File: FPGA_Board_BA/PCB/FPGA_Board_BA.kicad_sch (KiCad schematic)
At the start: 4 parts

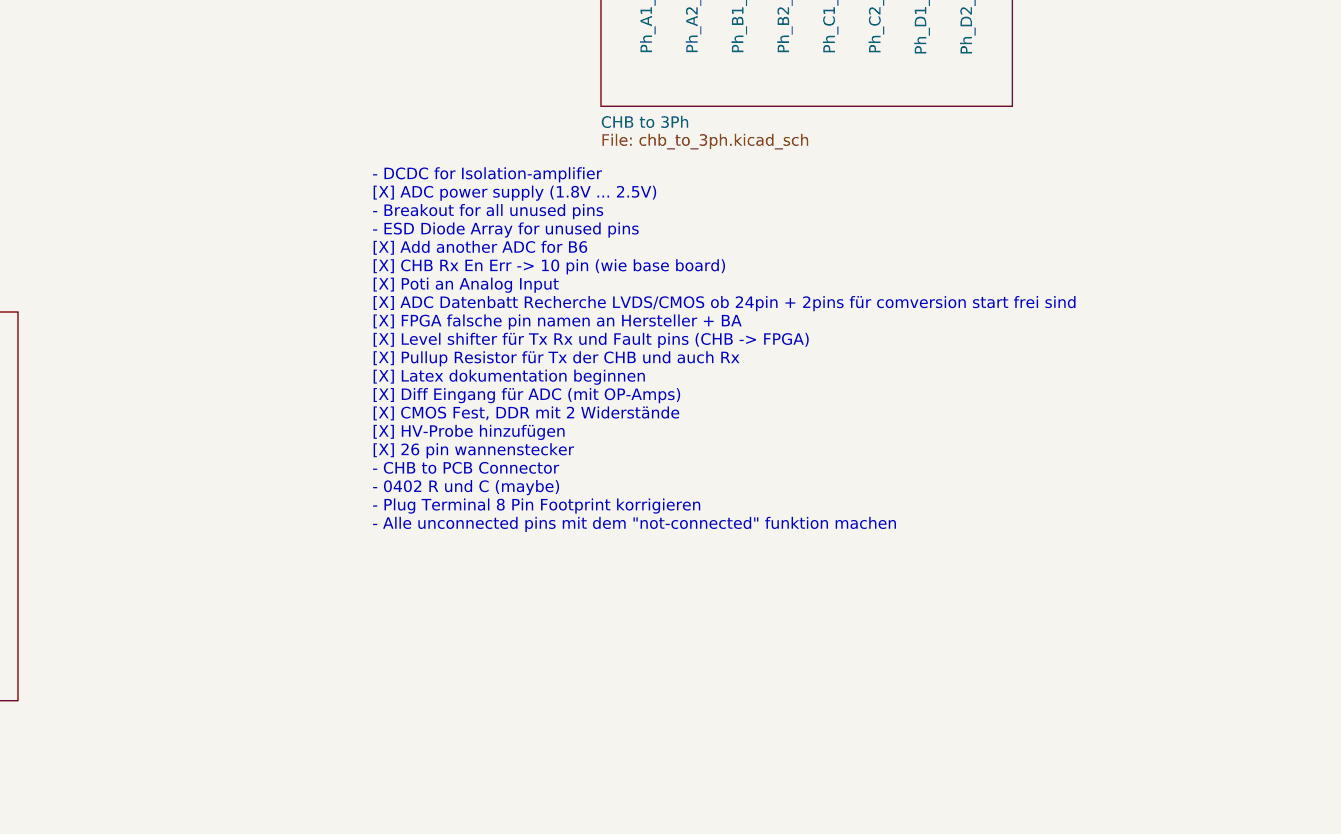
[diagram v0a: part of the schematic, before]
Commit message: Besprechung mit Leo
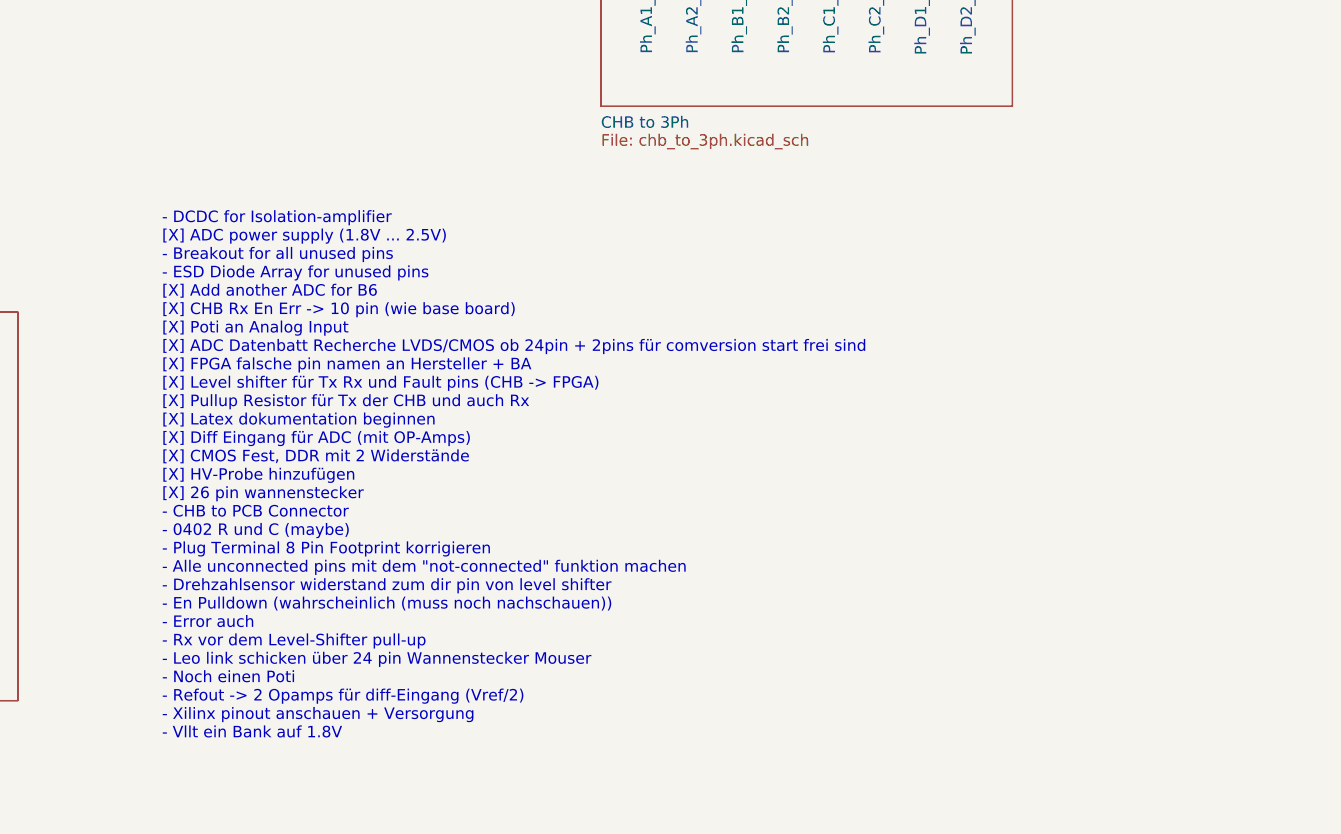
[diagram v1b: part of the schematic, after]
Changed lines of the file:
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@@
 	(generator_version "9.0")
 	(paper "A3")
-	(text "- DCDC for Isolation-amplifier\n[X] ADC power supply (1.8V ... 2.5V)\n- Breakout for all unused pins\n- ESD Diode Array for unused pins\n[X] Add another ADC for B6\n[X] CHB Rx En Err -> 10 pin (wie base board)\n[X] Poti an Analog Input\n[X] ADC Datenbatt Recherche LVDS/CMOS ob 24pin + 2pins für comversion start frei sind\n[X] FPGA falsche pin namen an Hersteller + BA \n[X] Level shifter für Tx Rx und Fault pins (CHB -> FPGA)\n[X] Pullup Resistor für Tx der CHB und auch Rx\n[X] Latex dokumentation beginnen\n[X] Diff Eingang für ADC (mit OP-Amps)\n[X] CMOS Fest, DDR mit 2 Widerstände\n[X] HV-Probe hinzufügen\n[X] 26 pin wannenstecker\n- CHB to PCB Connector \n- 0402 R und C (maybe)\n- Plug Terminal 8 Pin Footprint korrigieren\n- Alle unconnected pins mit dem \"not-connected\" funktion machen"
+	(text "- DCDC for Isolation-amplifier\n[X] ADC power supply (1.8V ... 2.5V)\n- Breakout for all unused pins\n- ESD Diode Array for unused pins\n[X] Add another ADC for B6\n[X] CHB Rx En Err -> 10 pin (wie base board)\n[X] Poti an Analog Input\n[X] ADC Datenbatt Recherche LVDS/CMOS ob 24pin + 2pins für comversion start frei sind\n[X] FPGA falsche pin namen an Hersteller + BA \n[X] Level shifter für Tx Rx und Fault pins (CHB -> FPGA)\n[X] Pullup Resistor für Tx der CHB und auch Rx\n[X] Latex dokumentation beginnen\n[X] Diff Eingang für ADC (mit OP-Amps)\n[X] CMOS Fest, DDR mit 2 Widerstände\n[X] HV-Probe hinzufügen\n[X] 26 pin wannenstecker\n- CHB to PCB Connector \n- 0402 R und C (maybe)\n- Plug Terminal 8 Pin Footprint korrigieren\n- Alle unconnected pins mit dem \"not-connected\" funktion machen\n- Drehzahlsensor widerstand zum dir pin von level shifter\n- En Pulldown (wahrscheinlich (muss noch nachschauen))\n- Error auch\n- Rx vor dem Level-Shifter pull-up\n- Leo link schicken über 24 pin Wannenstecker Mouser\n- Noch einen Poti \n- Refout -> 2 Opamps für diff-Eingang (Vref/2)\n- Xilinx pinout anschauen + Versorgung\n- Vllt ein Bank auf 1.8V"
 		(exclude_from_sim no)
-		(at 302.26 230.378 0)
+		(at 278.892 244.348 0)
 		(effects
 			(font

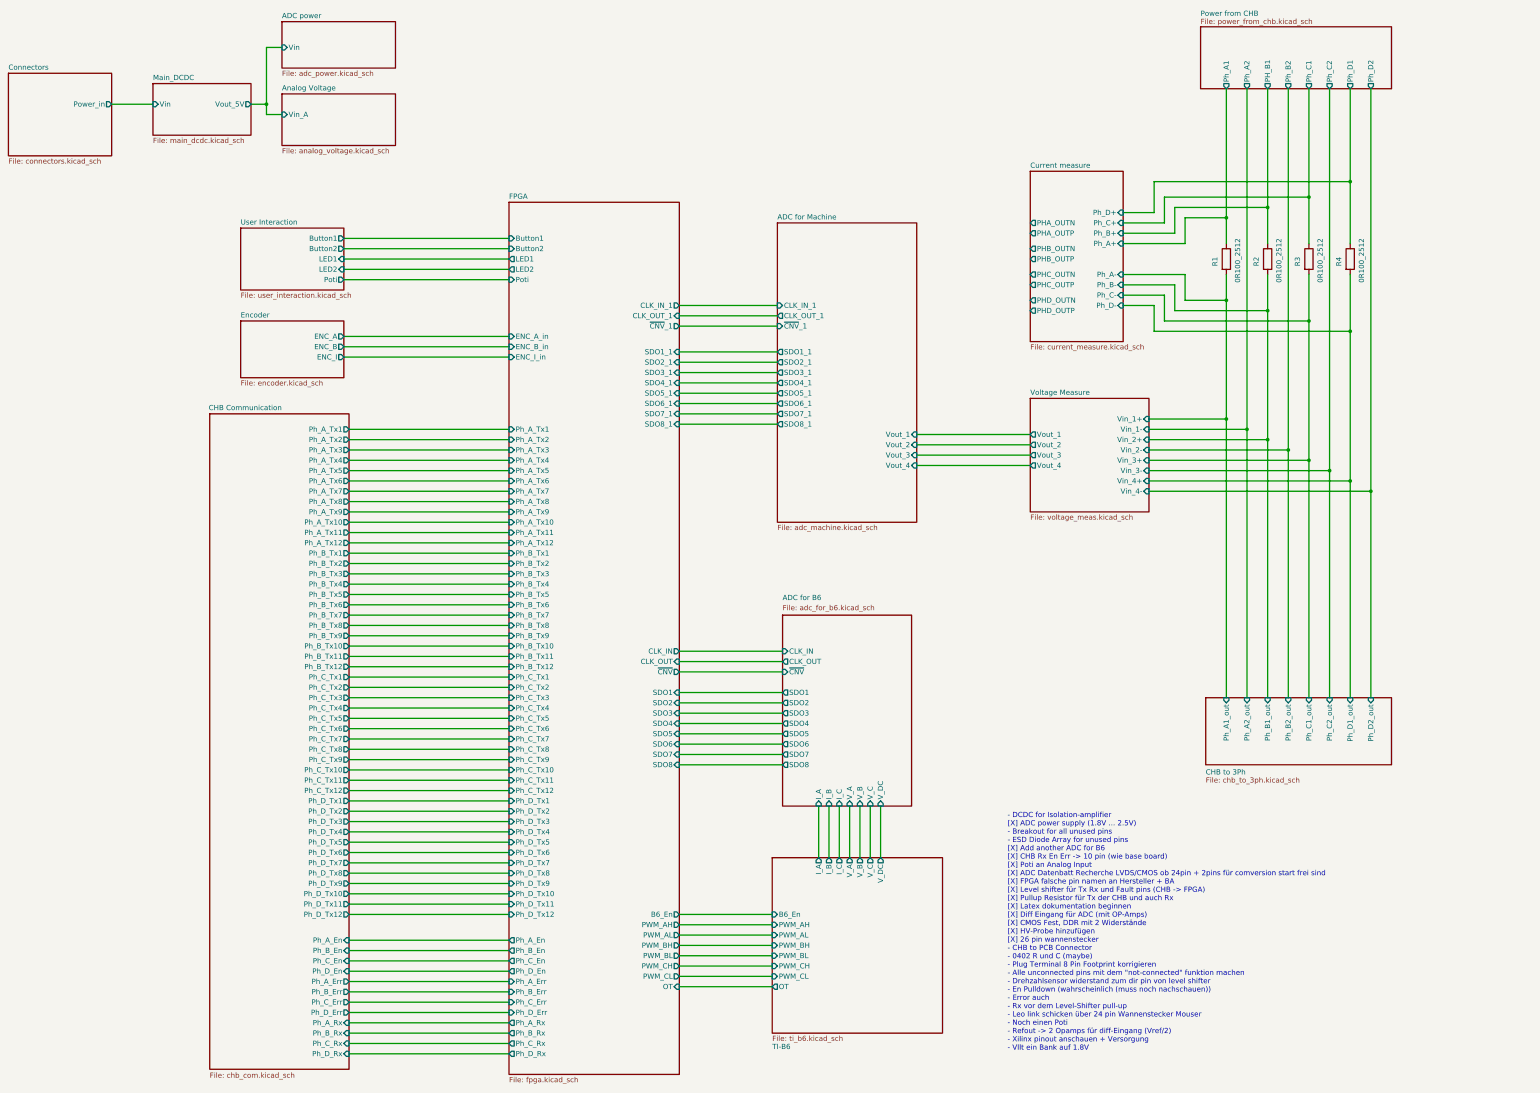
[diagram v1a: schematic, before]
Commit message: 22.11
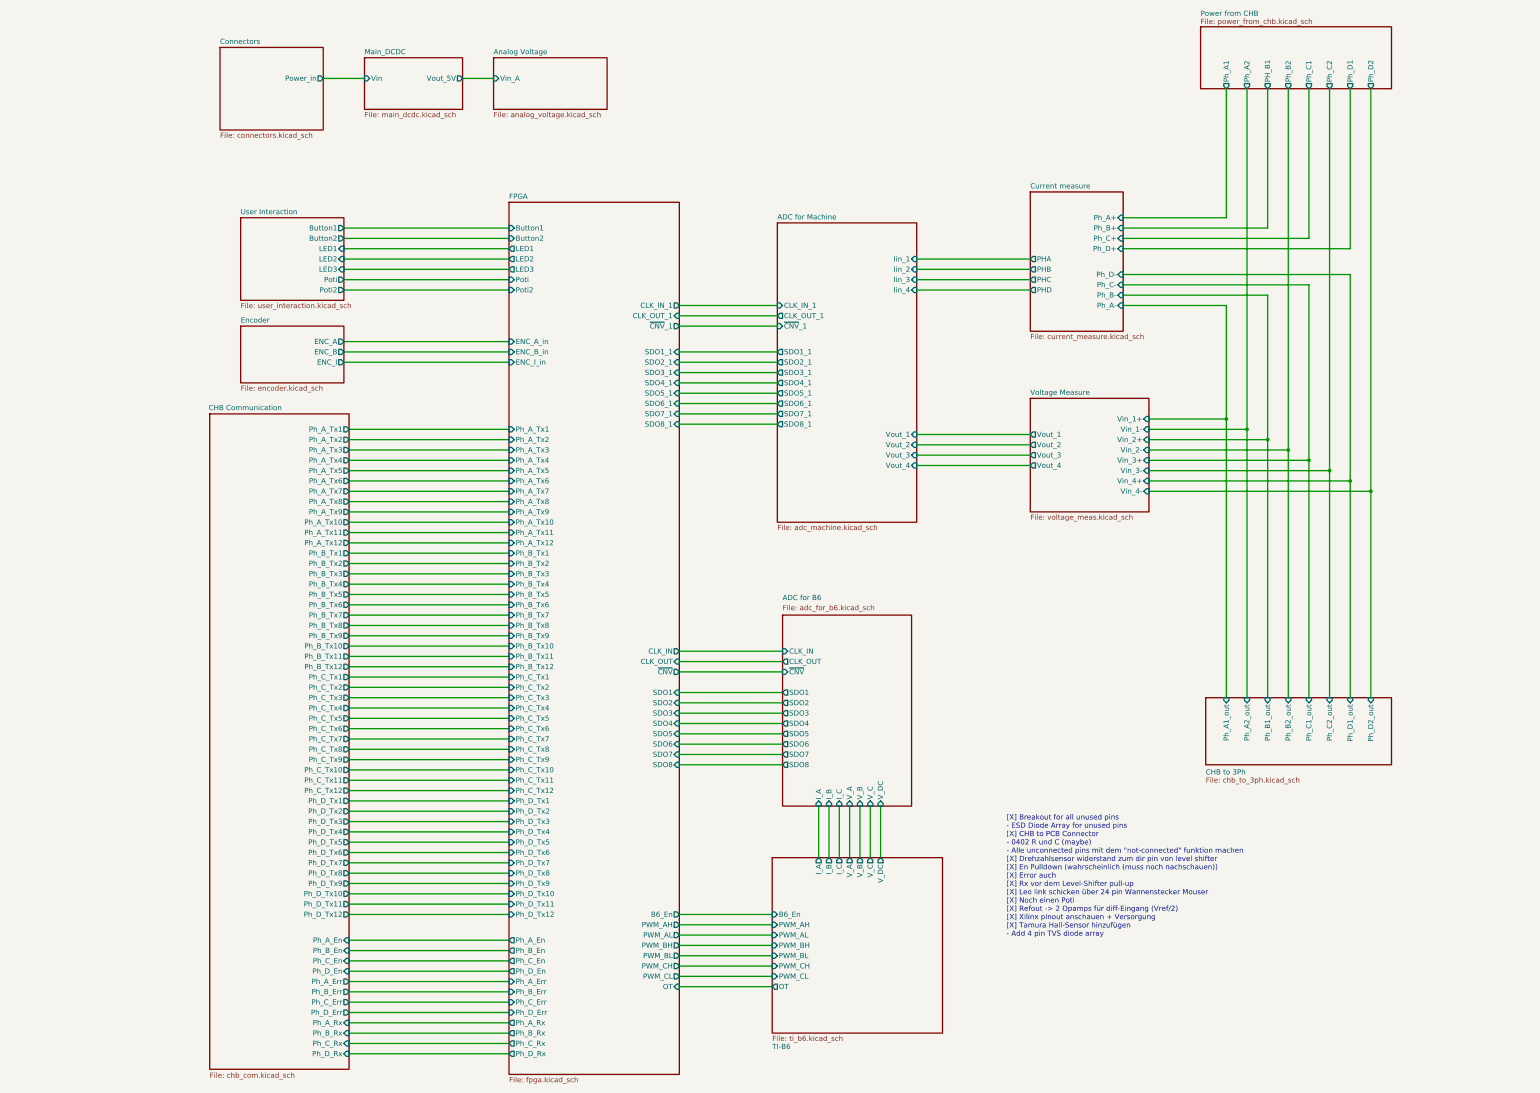
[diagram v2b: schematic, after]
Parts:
- removed R1, R2, R3, R4: 0R100_2512, Resistor_SMD:R_2512_6332Metric_Pad1.40x3.35mm_HandSolder, symbol MYLIB_R:0R100_2512
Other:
- removed sheet ADC power
- sheet ADC for Machine ports: added Iin_1, Iin_2, Iin_3, Iin_4; removed none
- sheet Current measure ports: added PHA, PHB, PHC, PHD; removed PHA_OUTN, PHA_OUTP, PHB_OUTN, PHB_OUTP, PHC_OUTN, PHC_OUTP, PHD_OUTN, PHD_OUTP
- sheet FPGA ports: added LED3, Poti2; removed none
- sheet User Interaction ports: added LED3, Poti2; removed none
- note added: "[X] Breakout for all unused pins - ESD Diode Array for unused pins [X] CHB to PCB Connector - 0402 R und C (maybe) - Alle unconnected pins mit dem "not-connected" funktion machen [X] Drehzahlsensor widerstand zum dir pin von level shifter [X] En Pulldown (wahrscheinlich (muss noch nachschauen)) [X] Error auch [X] Rx vor dem Level-Shifter pull-up [X] Leo link schicken über 24 pin Wannenstecker Mou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"
- note removed: "- DCDC for Isolation-amplifier [X] ADC power supply (1.8V ... 2.5V) - Breakout for all unused pins - ESD Diode Array for unused pins [X] Add another ADC for B6 [X] CHB Rx En Err -> 10 pin (wie base board) [X] Poti an Analog Input [X] ADC Datenbatt Recherche LVDS/CMOS ob 24pin + 2pins für comversion start frei sind [X] FPGA falsche pin namen an Hersteller + BA [X] Level shifter für Tx Rx und Fault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"
